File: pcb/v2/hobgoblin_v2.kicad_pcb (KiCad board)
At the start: 2 copper layers, 160 x 115 mm, 56 parts, among them J1 5V, J2 RC2014EXT1, J3 RC2014EXT2, J4 MINIUSB, SW1 RESET, SW2 ROMBNK, SW3 USBUART, U1 74LS32, U10 MC68B50, U2 74LS14, U3 Z80CPU, U4 GAL16V8/IO, U5 FT232RL, U6 628128, U7 74HCT00, U8 SST39SF010, U9 GAL16V8/MEM, X1 10MHz, X2 7.3728MHz

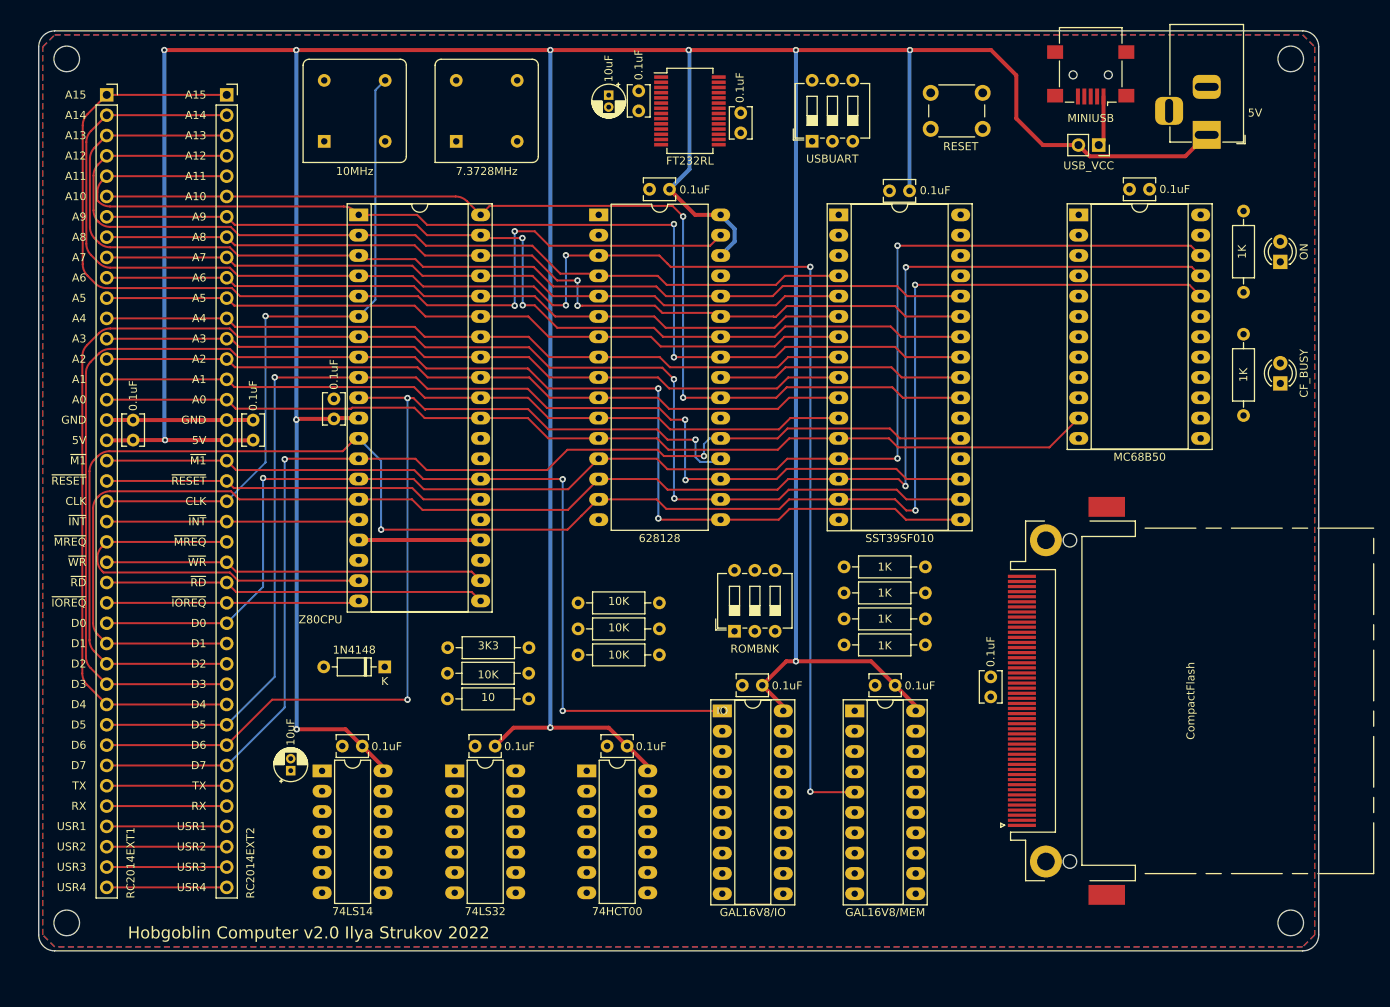
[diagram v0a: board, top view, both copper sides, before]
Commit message: PCB layout in progress
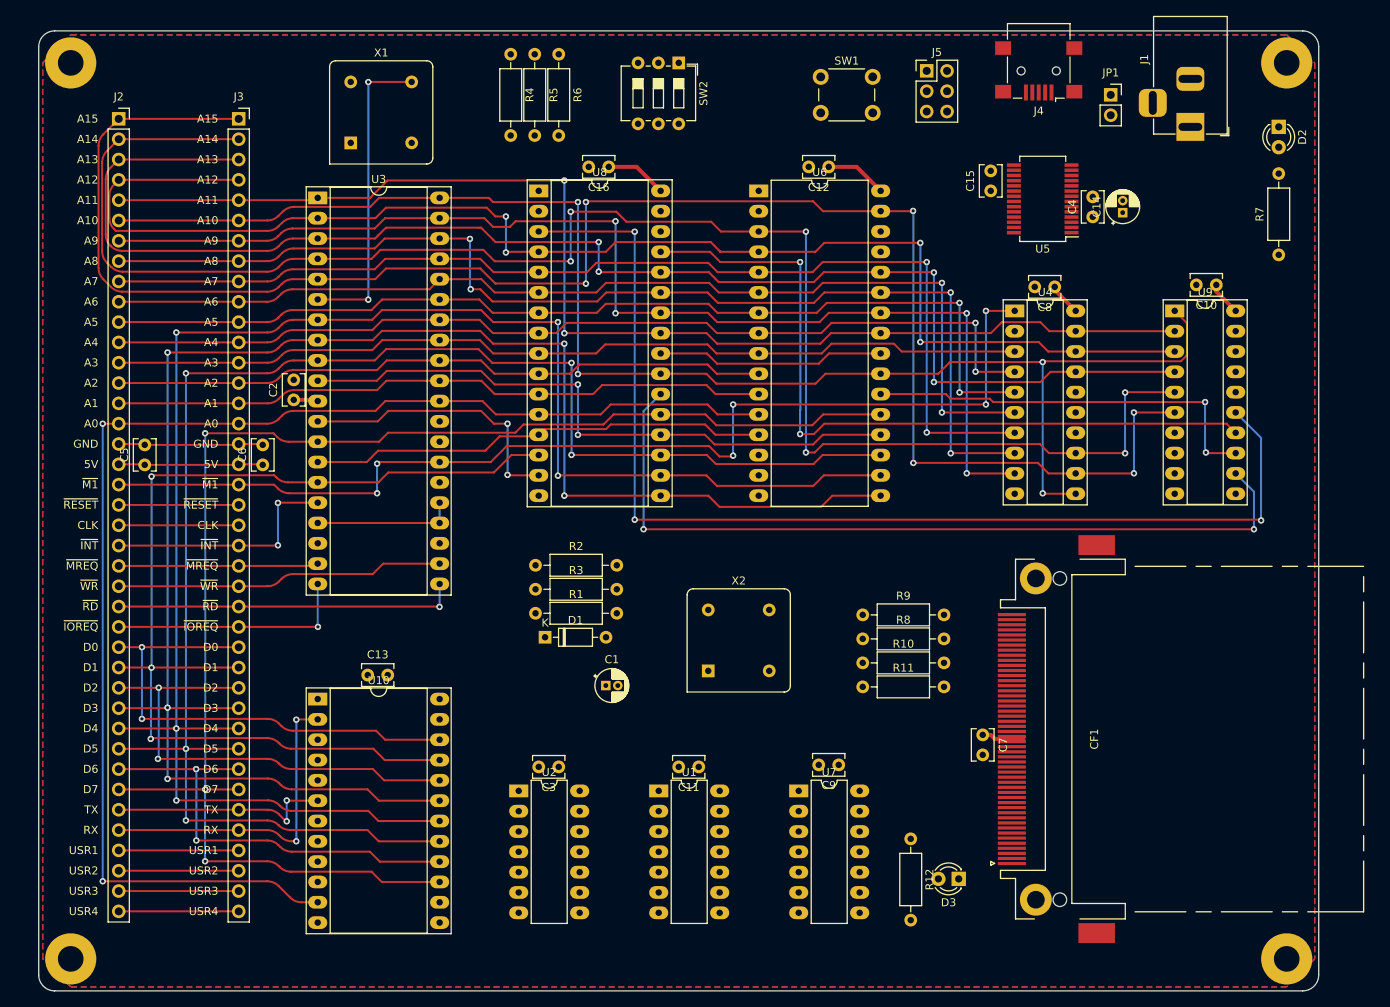
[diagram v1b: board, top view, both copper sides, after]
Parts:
- removed REF** (x4): M3, MountingHole:MountingHole_3.2mm_M3
- removed SW3: USBUART, Button_Switch_THT:SW_DIP_SPSTx03_Slide_6.7x9.18mm_W7.62mm_P2.54mm_LowProfile
- added J5: USBUART, Connector_PinHeader_2.54mm:PinHeader_2x03_P2.54mm_Vertical, F.Cu at (131.0, 25.0)
- added REF1: hole1, MountingHole:MountingHole_3.2mm_M3_Pad, F.Cu at (24.0, 24.0)
- added REF1: hole3, MountingHole:MountingHole_3.2mm_M3_Pad, F.Cu at (24.0, 136.0)
- added REF1: hole4, MountingHole:MountingHole_3.2mm_M3_Pad, F.Cu at (176.0, 136.0)
- added REF1: hole2, MountingHole:MountingHole_3.2mm_M3_Pad, F.Cu at (176.0, 24.0)
- moved U10 112.7 mm to (54.9, 103.5)
- moved C8 102.0 mm to (147.0, 52.0), turned to 180 degrees
- moved C4 99.8 mm to (151.8, 43.2), turned to 90 degrees
- moved C6 87.8 mm to (48.0, 74.2), turned to 90 degrees
- moved R6 76.1 mm to (85.0, 22.9), turned to -90 degrees
- moved R12 75.6 mm to (129.0, 121.0)
- moved D3 73.8 mm to (135.0, 126.0), turned to 180 degrees
- moved R5 73.5 mm to (82.0, 22.9), turned to -90 degrees
- moved X2 73.3 mm to (103.7, 100.0)
- moved SW2 71.4 mm to (100.0, 24.0), turned to -90 degrees
- moved R4 71.1 mm to (79.0, 22.9), turned to -90 degrees
- moved C5 69.8 mm to (33.2, 74.2), turned to 90 degrees
- moved C16 68.6 mm to (91.2, 37.0), turned to 180 degrees
- moved C14 65.9 mm to (155.5, 42.7), turned to 90 degrees
- moved U9 64.0 mm to (162.0, 55.0)
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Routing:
- net VCC: track 590.2 -> 68.0 mm, vias 11 -> 0
- net /ROM_A15: track 0.00 -> 141.2 mm, vias 0 -> 3
- net /D2: track 222.5 -> 95.4 mm, vias 3 -> 4
- net /~{ROM}: track 0.00 -> 102.0 mm, vias 0 -> 2
- net /ROM_A14: track 0.00 -> 94.9 mm, vias 0 -> 2
- net /A15: track 130.1 -> 222.9 mm, vias 2 -> 6
- net /D1: track 204.0 -> 135.1 mm, vias 2 -> 3
- net /D0: track 182.6 -> 119.7 mm, vias 3 -> 2
- net /A12: track 120.2 -> 174.8 mm, vias 0 -> 4
- net /A10: track 132.4 -> 184.9 mm, vias 2 -> 4
- net /~{RAM}: track 0.00 -> 51.1 mm, vias 0 -> 2
- net /D5: track 157.5 -> 204.6 mm, vias 3 -> 5
- net /A0: track 126.8 -> 169.7 mm, vias 0 -> 2
- net /A7: track 94.4 -> 136.5 mm, vias 0 -> 2
- net /D7: track 145.6 -> 186.0 mm, vias 2 -> 3
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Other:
- board size 160 x 115 mm -> 160 x 120 mm
- board text removed: "Hobgoblin Computer v2.0 Ilya Strukov 2022"
